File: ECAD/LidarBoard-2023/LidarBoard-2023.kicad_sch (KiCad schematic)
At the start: 17 parts, among them J1 Serial_Strategy, J2 Serial_Lidar, J3 Conn_01x03, J4 Oled, U1 Teensy3.2, U2 AMS1117-3.3

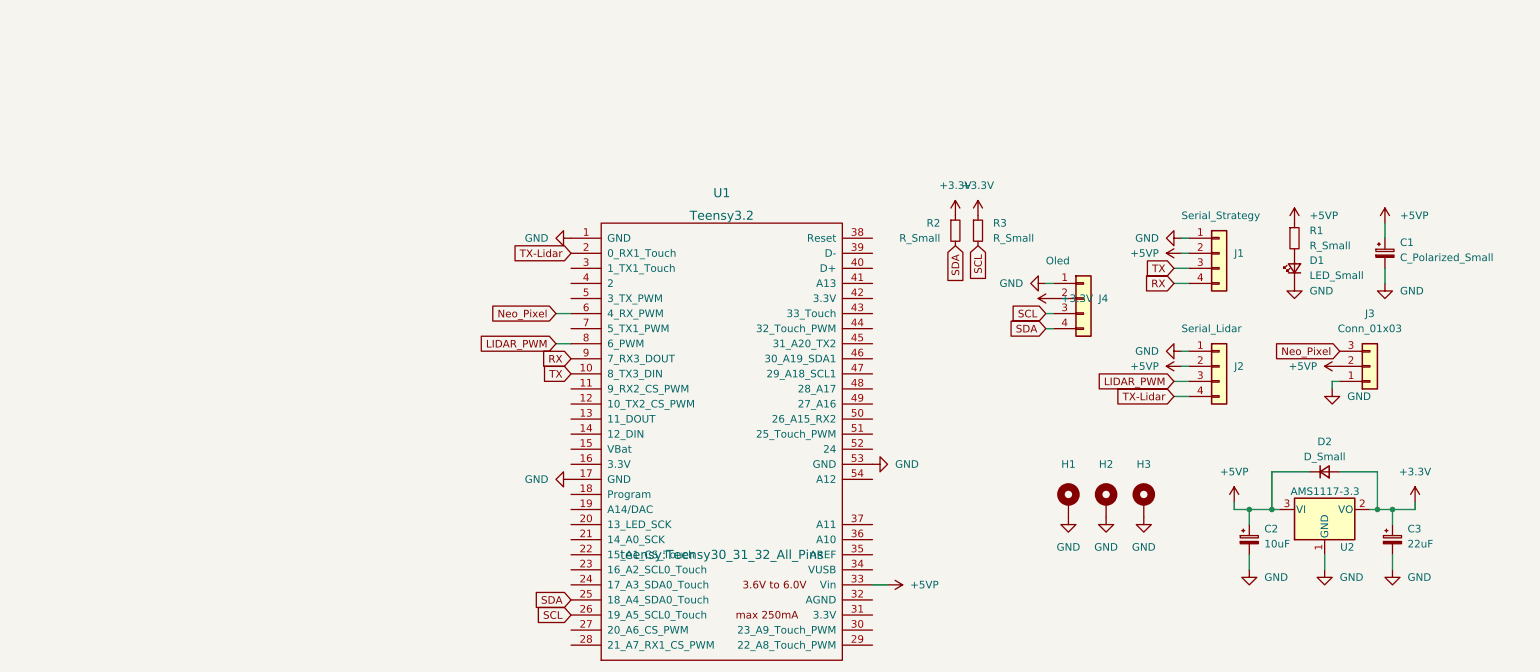
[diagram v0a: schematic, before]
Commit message: Change annotations
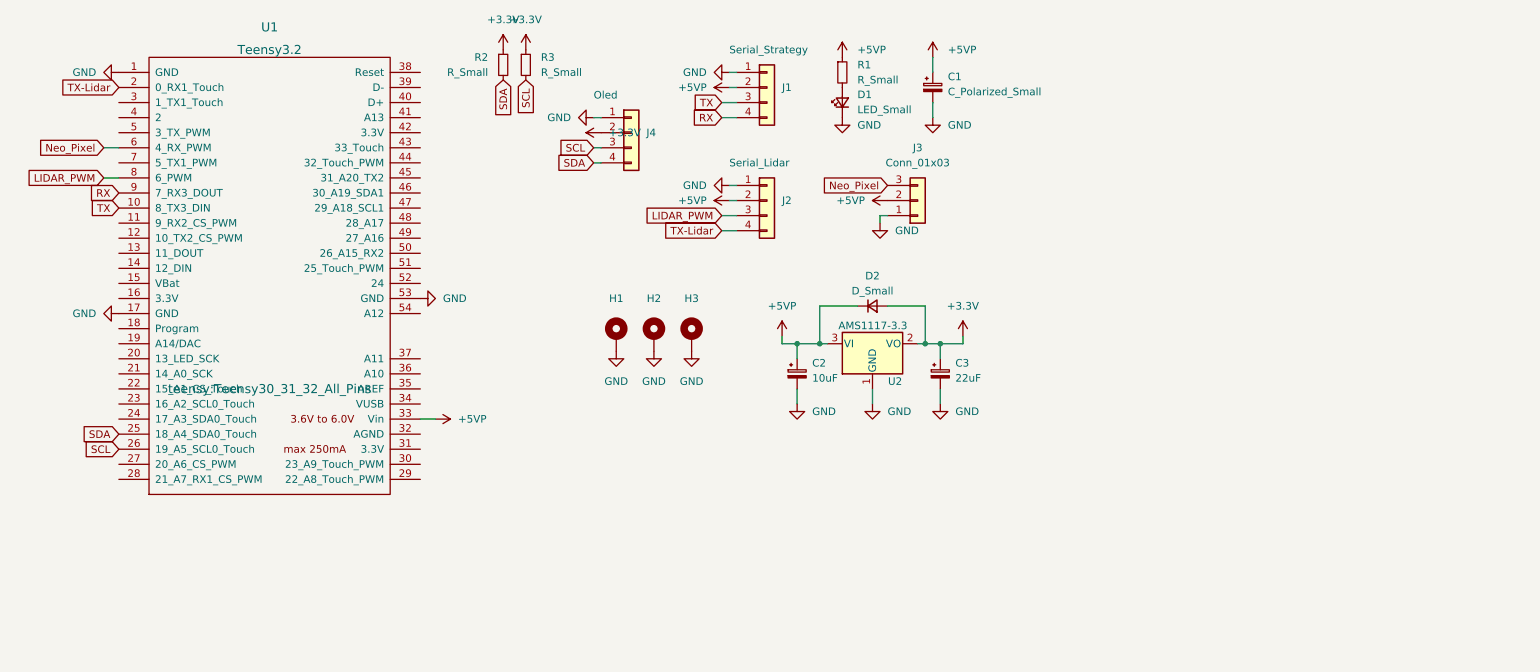
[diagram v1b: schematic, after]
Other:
- company: (none) -> Les Karibous
- title: (none) -> Lidar Board 2023
- moved on the sheet: C1, C2, C3, D1, D2, H1, H2, H3, J1, J2, J3, J4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
